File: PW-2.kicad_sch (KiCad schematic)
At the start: 10 parts, among them J1 Conn_01x02_Male, J2 Conn_01x02_Female, Q1 BSC025N08LS5

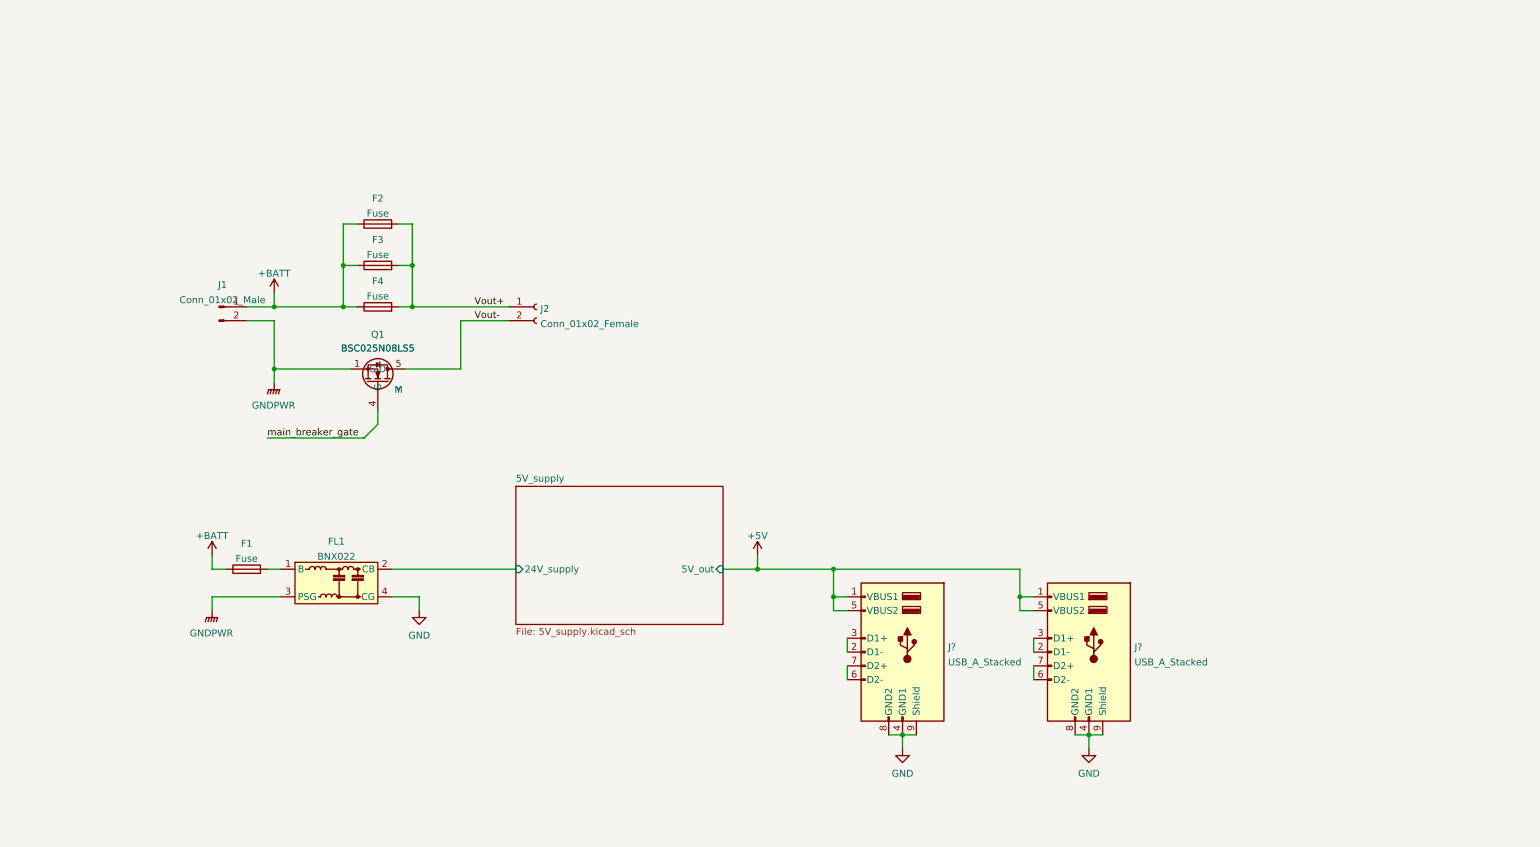
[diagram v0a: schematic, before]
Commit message: many
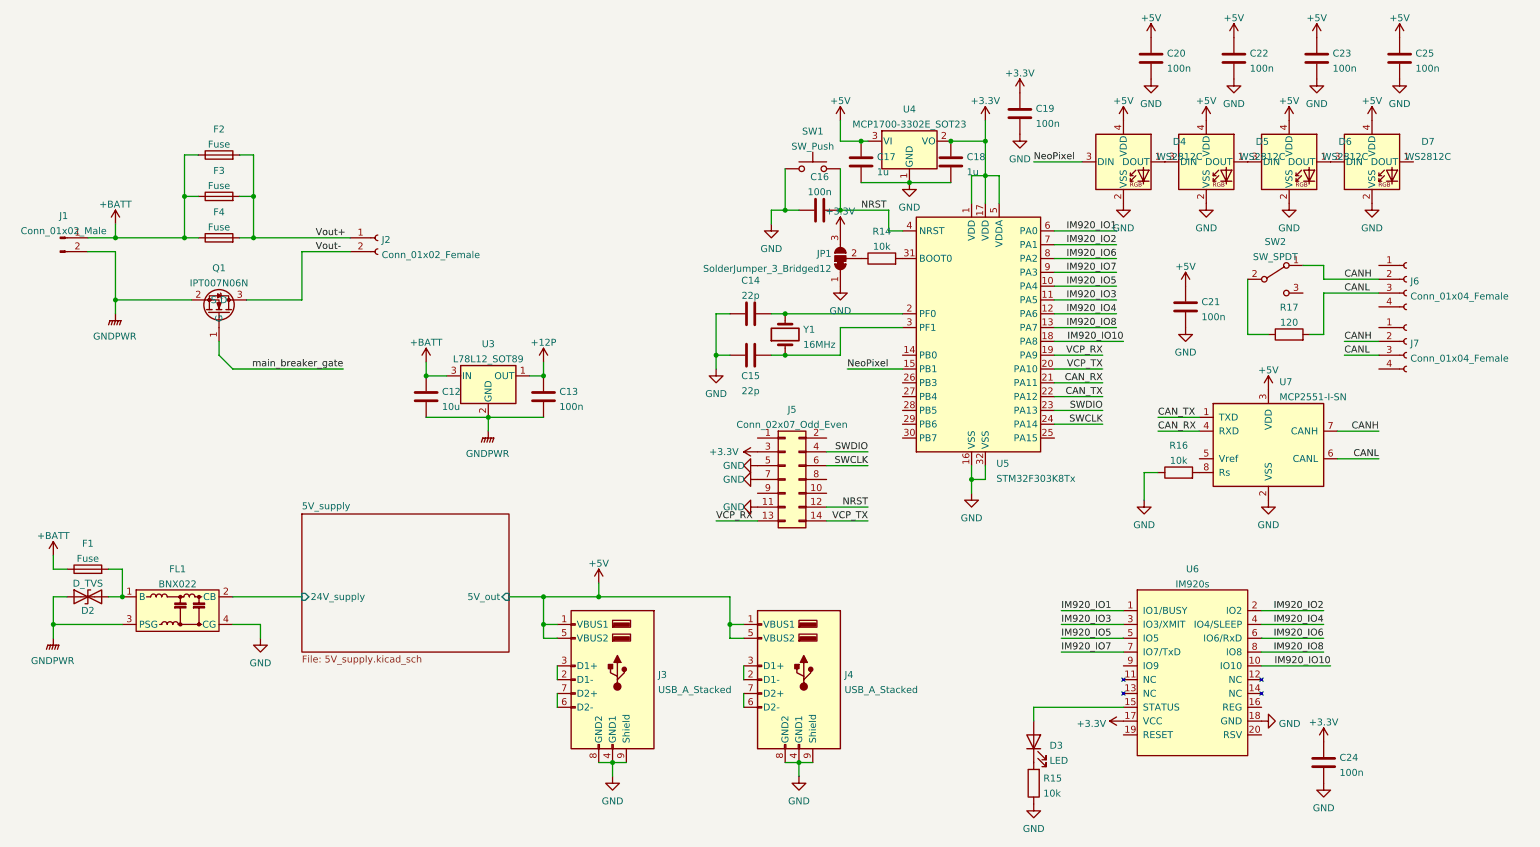
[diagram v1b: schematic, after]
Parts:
- removed Q1: BSC025N08LS5, Package_TO_SOT_SMD:TDSON-8-1, symbol Transistor_FET_additional:BSC025N08LS5
- added C12: 10u, Capacitor_SMD:C_0805_2012Metric, symbol Device:C
- added C13, C16, C19, C20, C21, C22, C23, C24, C25: 100n, Capacitor_SMD:C_0603_1608Metric, symbol Device:C
- added C14, C15: 22p, Capacitor_SMD:C_0603_1608Metric, symbol Device:C
- added C17, C18: 1u, Capacitor_SMD:C_0603_1608Metric, symbol Device:C
- added D2: D_TVS, Diode_SMD:D_SMA, symbol Device:D_TVS
- added D3: LED, Resistor_SMD:R_0603_1608Metric, symbol Device:LED
- added D4, D5, D6, D7: WS2812C, LED_additional:LED_2020Metric_WS2812C_2.0x2.0mm_P1.0mm, symbol LED_additional:WS2812C
- added J5: Conn_02x07_Odd_Even, Connector_PinHeader_1.27mm:PinHeader_2x07_P1.27mm_Vertical_SMD, symbol Connector_Generic:Conn_02x07_Odd_Even
- added J6, J7: Conn_01x04_Female, Connector_JST:JST_XA_S04B-XASK-1_1x04_P2.50mm_Horizontal, symbol Connector:Conn_01x04_Female
- added JP1: SolderJumper_3_Bridged12, Jumper:SolderJumper-3_P1.3mm_Bridged12_RoundedPad1.0x1.5mm, symbol Jumper:SolderJumper_3_Bridged12
- added Q1: IPT007N06N, Package_TO_SOT_SMD:Infineon_PG-HSOF-8-1_ThermalVias, symbol Transistor_FET_additional:IPT007N06N
- added R14, R15, R16: 10k, Resistor_SMD:R_0603_1608Metric, symbol Device:R
- added R17: 120, Resistor_SMD:R_0603_1608Metric, symbol Device:R
- added SW1: SW_Push, Button_Switch_additional:TVAF06-A020B-R, symbol Switch:SW_Push
- added SW2: SW_SPDT, Button_Switch_additional:IS-1245T-G, symbol Switch:SW_SPDT
- added U3: L78L12_SOT89, Package_TO_SOT_SMD:SOT-89-3, symbol Regulator_Linear:L78L12_SOT89
- added U4: MCP1700-3302E_SOT23, Package_TO_SOT_SMD:SOT-23, symbol Regulator_Linear:MCP1700-3302E_SOT23
- added U5: STM32F303K8Tx, Package_QFP:LQFP-32_7x7mm_P0.8mm, symbol MCU_ST_STM32F3:STM32F303K8Tx
- added U6: IM920s, interplan:IM920s, symbol interplan:IM920s
- added U7: MCP2551-I-SN, Package_SO:SOIC-8_3.9x4.9mm_P1.27mm, symbol Interface_CAN_LIN:MCP2551-I-SN
- added Y1: 16MHz, Crystal:Crystal_SMD_HC49-SD, symbol Device:Crystal
- F1, F2, F3, F4: footprint (none) -> Fuse_additional:Fuseholder_Keystone_3568
- gave numbers to parts that had none: 2
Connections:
- net +5V: now also C17.2, C20.2, C21.2, C22.2, C23.2, C25.2, D4.4 (VDD), D5.4 (VDD), D6.4 (VDD), D7.4 (VDD), U4.3 (VI), U7.3 (VDD)
- net +BATT: now also C12.1, U3.3 (IN)
- net GND: now also C14.1, C15.1, C16.1, C17.1, C18.1, C19.1, C20.1, C21.1, C22.1, C23.1, C24.1, C25.1, D4.2 (VSS), D5.2 (VSS), D6.2 (VSS), D7.2 (VSS), J5.11 (Pin_11), J5.5 (Pin_5), J5.7 (Pin_7), JP1.1 (A), R15.1, R16.1, SW1.1, U4.1 (GND), U5.16 (VSS), U5.32 (VSS), U6.18 (GND), U7.2 (VSS)
- net GNDPWR: now also C12.2, C13.1, D2.1 (A1), Q1.2 (S), U3.2 (GND)
- net Vout-: now also Q1.3 (D)
- net main_breaker_gate: now also Q1.1 (G)
- net at F1.2, FL1.1 (B): now also D2.2 (A2)
- new net: C15.2, U5.3 (PF1), Y1.1
- new net: D3.1 (K), R15.2
- new net: JP1.2 (C), R14.1
- new net: D5.1 (DOUT), D6.3 (DIN)
- new net: D4.1 (DOUT), D5.3 (DIN)
- new net: D3.2 (A), U6.15 (STATUS)
- new net: R14.2, U5.31 (BOOT0)
- new net: R16.2, U7.8 (Rs)
- new net: R17.1, SW2.2 (B)
- new net: C14.2, U5.2 (PF0), Y1.2
- new net: D6.1 (DOUT), D7.3 (DIN)
- new net +12P: C13.2, U3.1 (OUT)
- new net +3V3: C18.2, C19.2, C24.2, J5.3 (Pin_3), JP1.3 (B), U4.2 (VO), U5.1 (VDD), U5.17 (VDD), U5.5 (VDDA), U6.17 (VCC)
- new net CANH: J6.2 (Pin_2), J7.2 (Pin_2), SW2.1 (A), U7.7 (CANH)
- new net CANL: J6.3 (Pin_3), J7.3 (Pin_3), R17.2, U7.6 (CANL)
- new net CAN_RX: U5.21 (PA11), U7.4 (RXD)
- new net CAN_TX: U5.22 (PA12), U7.1 (TXD)
- new net IM920_IO1: U5.6 (PA0), U6.1 (IO1/BUSY)
- new net IM920_IO10: U5.18 (PA8), U6.10 (IO10)
- new net IM920_IO2: U5.7 (PA1), U6.2 (IO2)
- new net IM920_IO3: U5.11 (PA5), U6.3 (IO3/XMIT)
- new net IM920_IO4: U5.12 (PA6), U6.4 (IO4/SLEEP)
- new net IM920_IO5: U5.10 (PA4), U6.5 (IO5)
- new net IM920_IO6: U5.8 (PA2), U6.6 (IO6/RxD)
- new net IM920_IO7: U5.9 (PA3), U6.7 (IO7/TxD)
- new net IM920_IO8: U5.13 (PA7), U6.8 (IO8)
- new net NRST: C16.2, J5.12 (Pin_12), SW1.2, U5.4 (NRST)
- new net NeoPixel: D4.3 (DIN), U5.15 (PB1)
- new net SWCLK: J5.6 (Pin_6), U5.24 (PA14)
- new net SWDIO: J5.4 (Pin_4), U5.23 (PA13)
- new net VCP_RX: J5.13 (Pin_13), U5.19 (PA9)
- new net VCP_TX: J5.14 (Pin_14), U5.20 (PA10)
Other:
- moved on the sheet: F1, F2, F3, F4, FL1, J1, J2, J3, J4
